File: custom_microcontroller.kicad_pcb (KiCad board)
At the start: 2 copper layers, 27.9 x 47.8 mm, 29 parts, among them J1 Conn_01x05_Male, J2 Conn_01x02_Male, J3 Conn_01x08_Male, J4 Conn_01x02_Male, J5 Conn_01x02_Male, J6 Conn_01x06_Male, J7 Conn_01x02_Male, U1 NCP1117ST33T3G, U2 STM32F042G6Ux, U3 SN65HVD233, Y1 Crystal_GND24

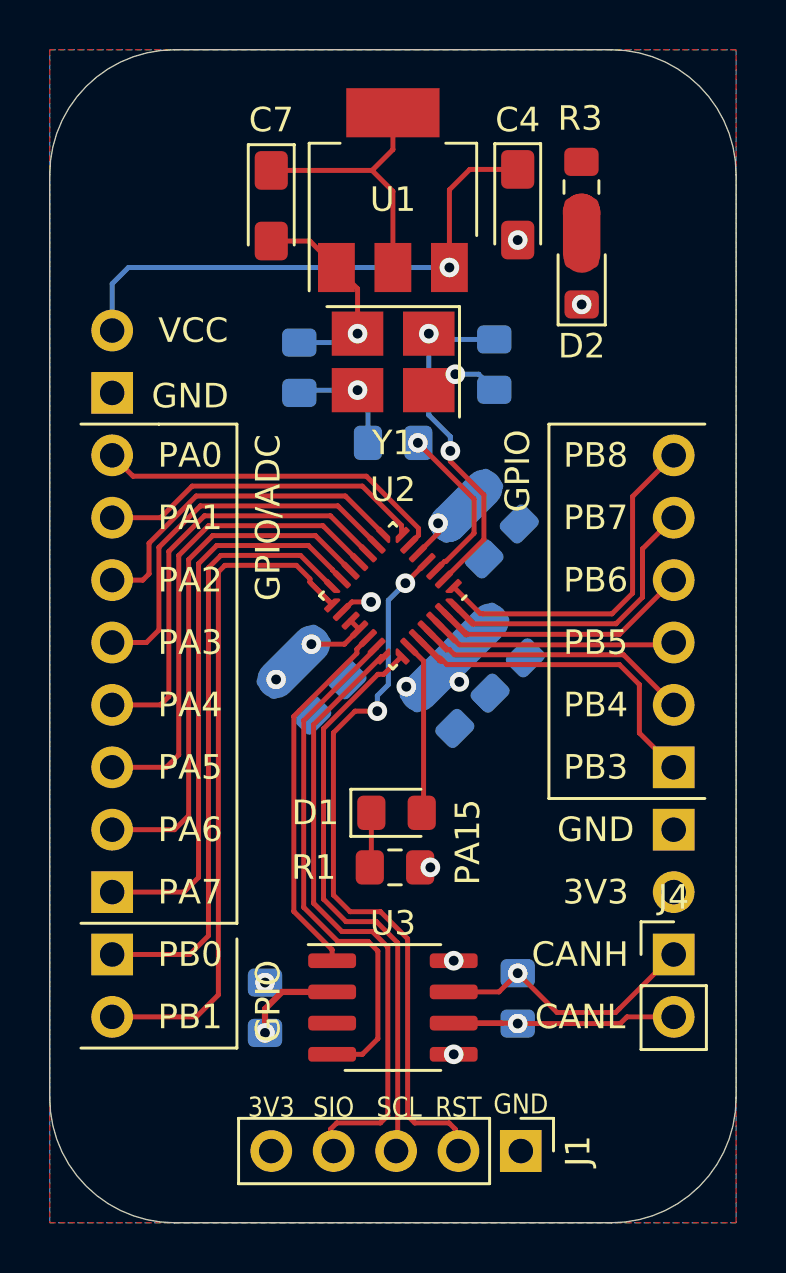
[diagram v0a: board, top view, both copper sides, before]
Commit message: single layer design
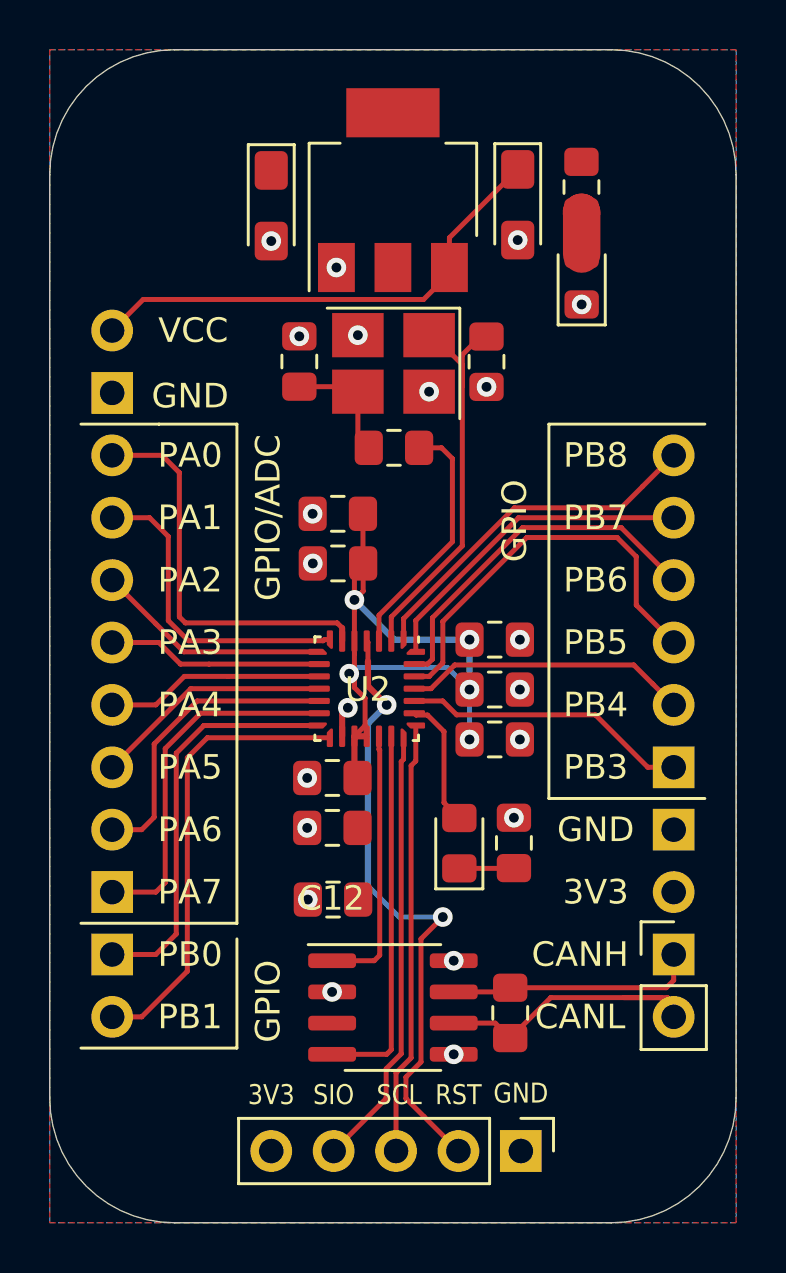
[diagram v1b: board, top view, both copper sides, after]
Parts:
- added G***: LOGO, memes:little_creatures, B.Cu at (138.6, 116.6)
- C1, C10, C11, C12, C2, C3, C5, C6, C8, C9, R2, R4: moved to F.Cu
- moved C6 6.67 mm to (136.2, 125.6), turned to 180 degrees
- moved C1 5.54 mm to (136.0, 138.4), turned to 180 degrees
- moved C8 5.30 mm to (136.2, 127.6), turned to 180 degrees
- moved C12 5.20 mm to (136.0, 141.3), turned to 180 degrees
- moved R1 4.94 mm to (143.4, 139.0), turned to 270 degrees
- moved C5 4.72 mm to (136.0, 136.3), turned to 180 degrees
- moved U2 3.93 mm to (137.4, 132.7), turned to 270 degrees
- moved D1 2.84 mm to (141.1, 139.0), turned to 90 degrees
- moved C9 2.63 mm to (142.6, 134.8), turned to 0 degrees
- moved C11 1.08 mm to (142.6, 132.7), turned to 0 degrees
- moved R4 0.67 mm to (143.2, 145.9)
- moved C10 0.52 mm to (142.6, 130.7), turned to 0 degrees
- moved C2 0.34 mm to (142.2, 119.4)
- moved C3 0.25 mm to (134.6, 119.4)
- moved R2 0.21 mm to (138.5, 122.9)
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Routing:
- net GND: track 17.6 -> 1.26 mm, vias 9 -> 21
- net /PB1: track 28.6 -> 18.7 mm
- net /PA5: track 19.5 -> 9.75 mm
- net /PA6: track 21.4 -> 12.3 mm
- net /PA4: track 17.7 -> 8.91 mm
- net /PA7: track 23.3 -> 14.6 mm
- net /SWDIO: track 25.6 -> 18.1 mm
- net /PA3: track 15.7 -> 8.79 mm
- net /PB5: track 10.2 -> 16.8 mm
- net /CAN_RX: track 21.3 -> 15.2 mm
- net /SWCLK: track 23.8 -> 17.9 mm
- net /NRST: track 29.8 -> 25.5 mm
- net /PA2: track 14.6 -> 10.3 mm
- net /PB6: track 10.7 -> 14.7 mm
- net /CAN_TX: track 15.0 -> 11.0 mm
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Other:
- board text added: "An STM32F042 Microcontroller with a built in CAN transceiver and CANH + CANL outputs."
- board text added: "SmolBoi.exe V2.0.0"
- board text added: "chenry was here"
- board text removed: "PA15"
